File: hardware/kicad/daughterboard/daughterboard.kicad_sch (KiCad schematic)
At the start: 8 parts, among them J1 X6511FV-24-C85D32, J2 X6511FV-24-C85D32, U1 XDJK-0051-025, U2 BX-PM2.54-1-14PY, U3 BX-PM2.54-1-14PY

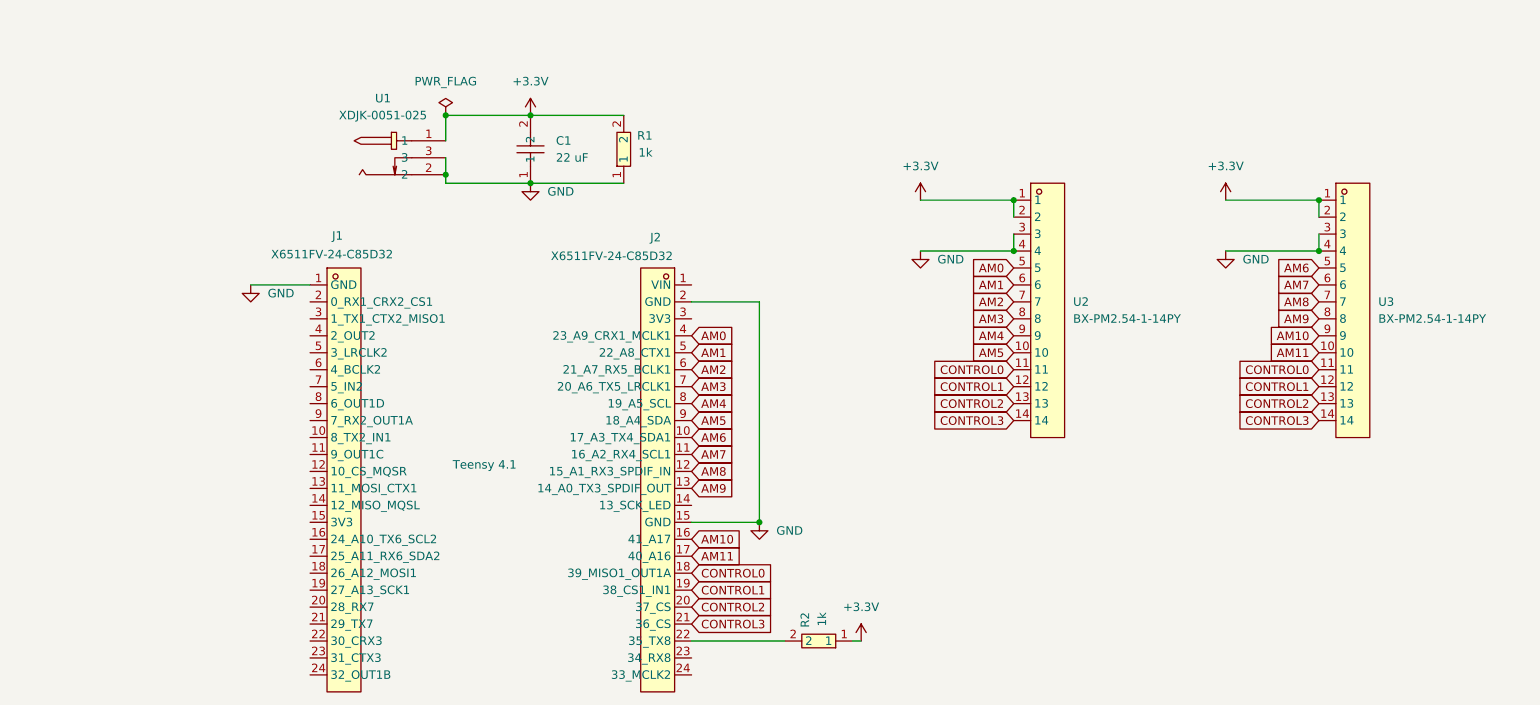
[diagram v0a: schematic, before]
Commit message: Ok
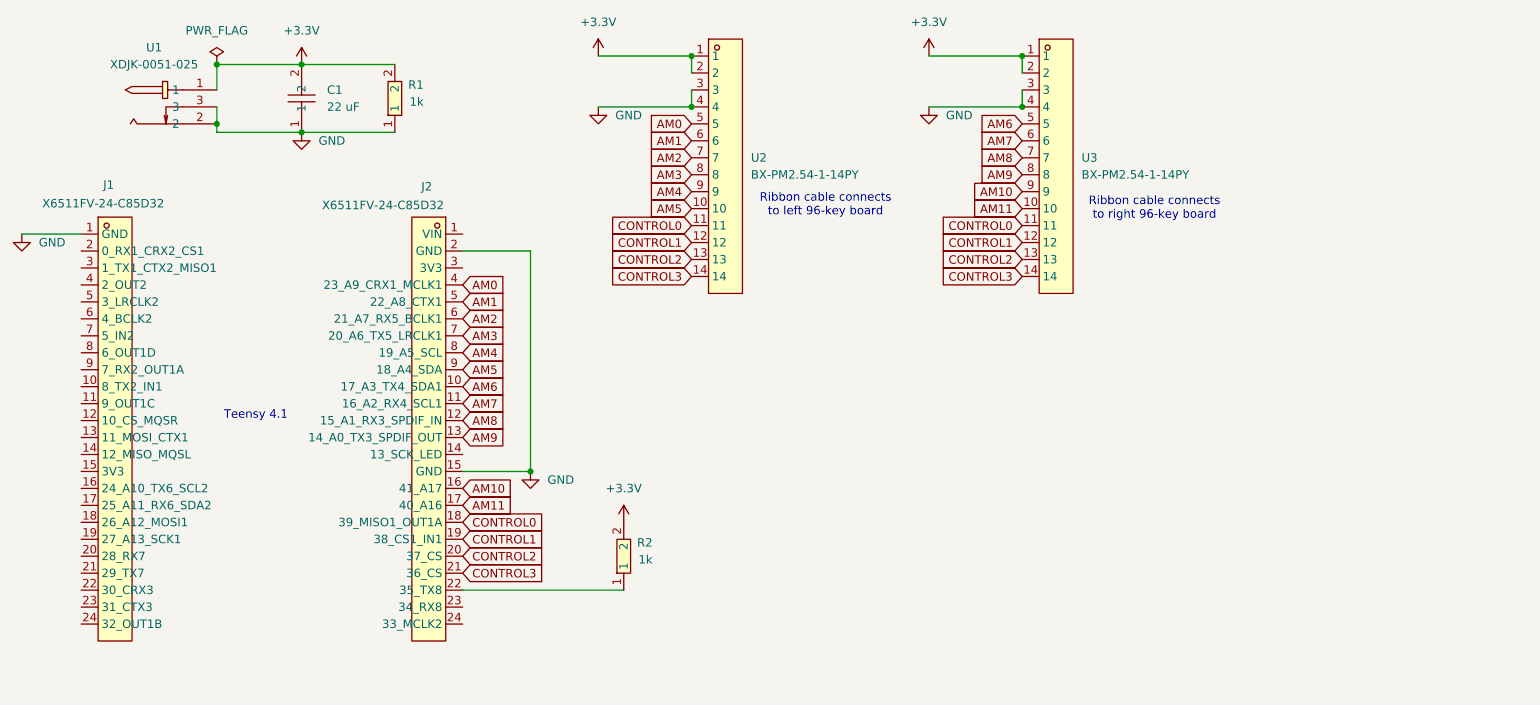
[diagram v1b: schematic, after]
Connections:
- net +3.3V: now also R2.2; no longer R2.1
- net at J2.22 (35_TX8): now also R2.1; no longer R2.2
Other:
- note added: "Ribbon cable connects to left 96-key board"
- note added: "Ribbon cable connects to right 96-key board"
- title: (none) -> https://github.com/DumpsterDoofus/keyboard_accordion
- moved on the sheet: C1, J1, J2, R1, R2, U1, U2, U3

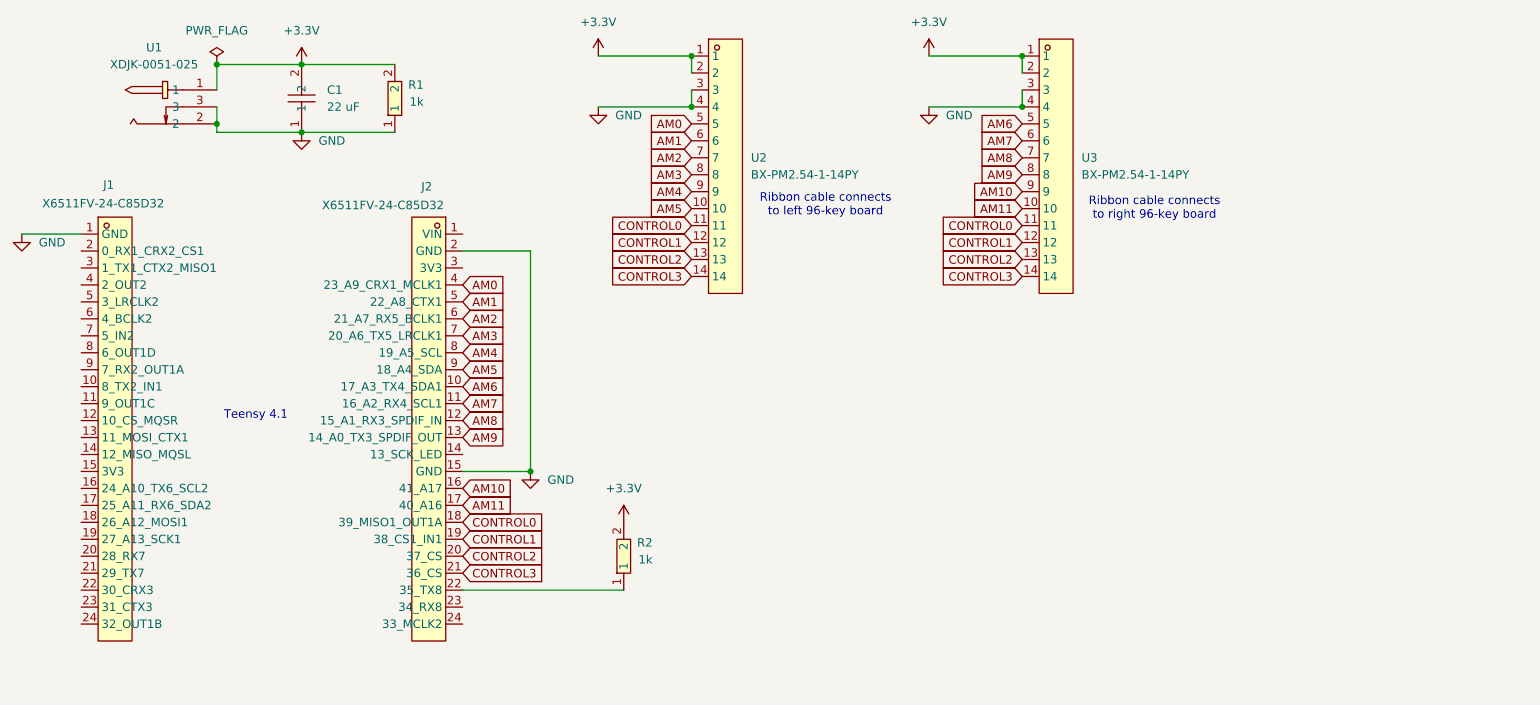
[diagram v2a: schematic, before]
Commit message: Ok
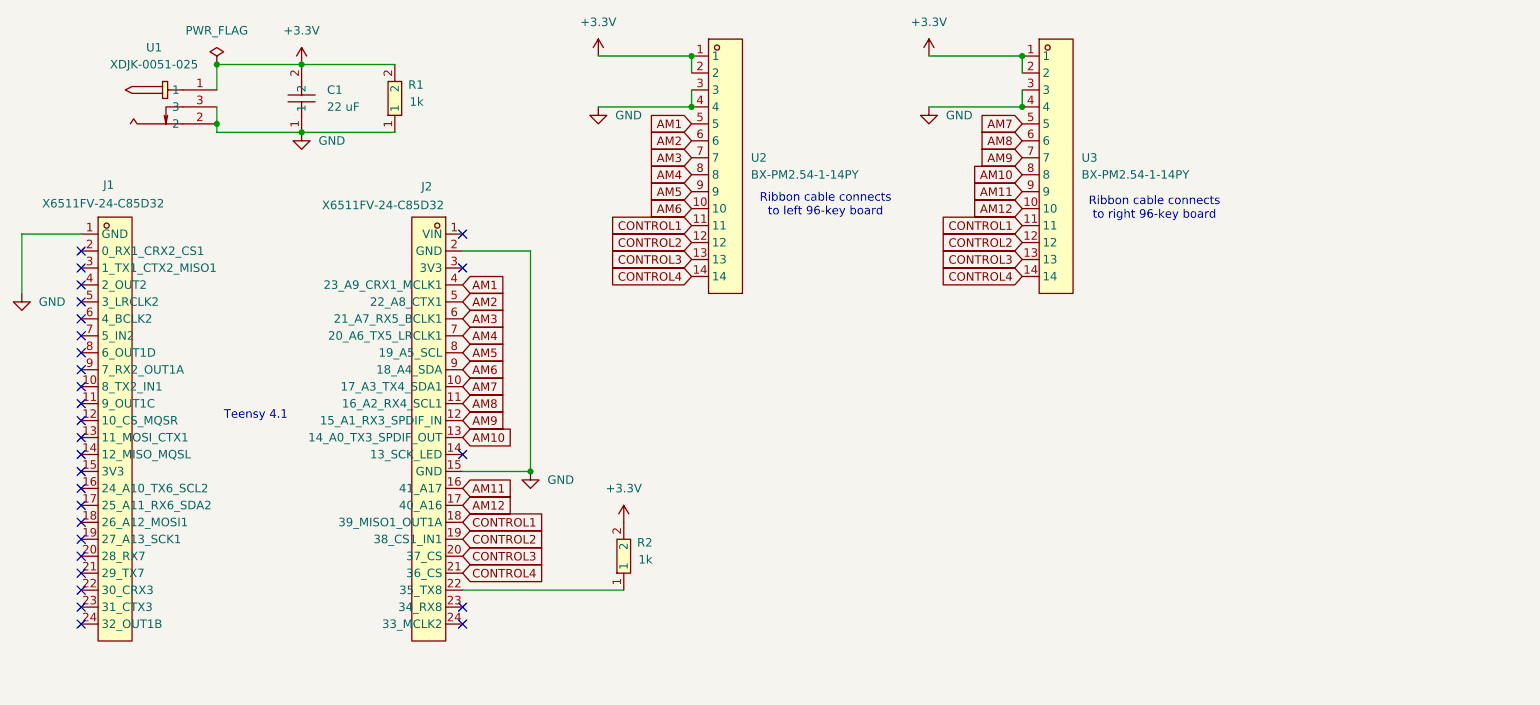
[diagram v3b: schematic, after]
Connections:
- net AM0 is gone; now on net AM1: J2.4 (23_A9_CRX1_MCLK1), U2.5
- net CONTROL0 is gone; now on net CONTROL1: J2.18 (39_MISO1_OUT1A), U2.11, U3.11
- net AM1: no longer J2.5 (22_A8_CTX1), U2.6
- net AM10: now also J2.13 (14_A0_TX3_SPDIF_OUT), U3.8; no longer J2.16 (41_A17), U3.9
- net AM11: now also J2.16 (41_A17), U3.9; no longer J2.17 (40_A16), U3.10
- net AM2: now also J2.5 (22_A8_CTX1), U2.6; no longer J2.6 (21_A7_RX5_BCLK1), U2.7
- net AM3: now also J2.6 (21_A7_RX5_BCLK1), U2.7; no longer J2.7 (20_A6_TX5_LRCLK1), U2.8
- net AM4: now also J2.7 (20_A6_TX5_LRCLK1), U2.8; no longer J2.8 (19_A5_SCL), U2.9
- net AM5: now also J2.8 (19_A5_SCL), U2.9; no longer J2.9 (18_A4_SDA), U2.10
- net AM6: now also J2.9 (18_A4_SDA), U2.10; no longer J2.10 (17_A3_TX4_SDA1), U3.5
- net AM7: now also J2.10 (17_A3_TX4_SDA1), U3.5; no longer J2.11 (16_A2_RX4_SCL1), U3.6
- net AM8: now also J2.11 (16_A2_RX4_SCL1), U3.6; no longer J2.12 (15_A1_RX3_SPDIF_IN), U3.7
- net AM9: now also J2.12 (15_A1_RX3_SPDIF_IN), U3.7; no longer J2.13 (14_A0_TX3_SPDIF_OUT), U3.8
- net CONTROL1: no longer J2.19 (38_CS1_IN1), U2.12, U3.12
- net CONTROL2: now also J2.19 (38_CS1_IN1), U2.12, U3.12; no longer J2.20 (37_CS), U2.13, U3.13
- net CONTROL3: now also J2.20 (37_CS), U2.13, U3.13; no longer J2.21 (36_CS), U2.14, U3.14
- new net AM12: J2.17 (40_A16), U3.10
- new net CONTROL4: J2.21 (36_CS), U2.14, U3.14
- no-connect marks 0 -> 28
